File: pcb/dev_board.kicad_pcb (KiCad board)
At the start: 6 copper layers, 45.1 x 41.2 mm, 38 parts, among them J1 Conn_02x13_Odd_Even, J2 Conn_02x13_Odd_Even, J4 Conn_01x05, SW1 SW_DIP_x03, SW2 ARM, U1 LPC, U2 MCP3202, U3 TLV75530PDBV, U6 TLV74311

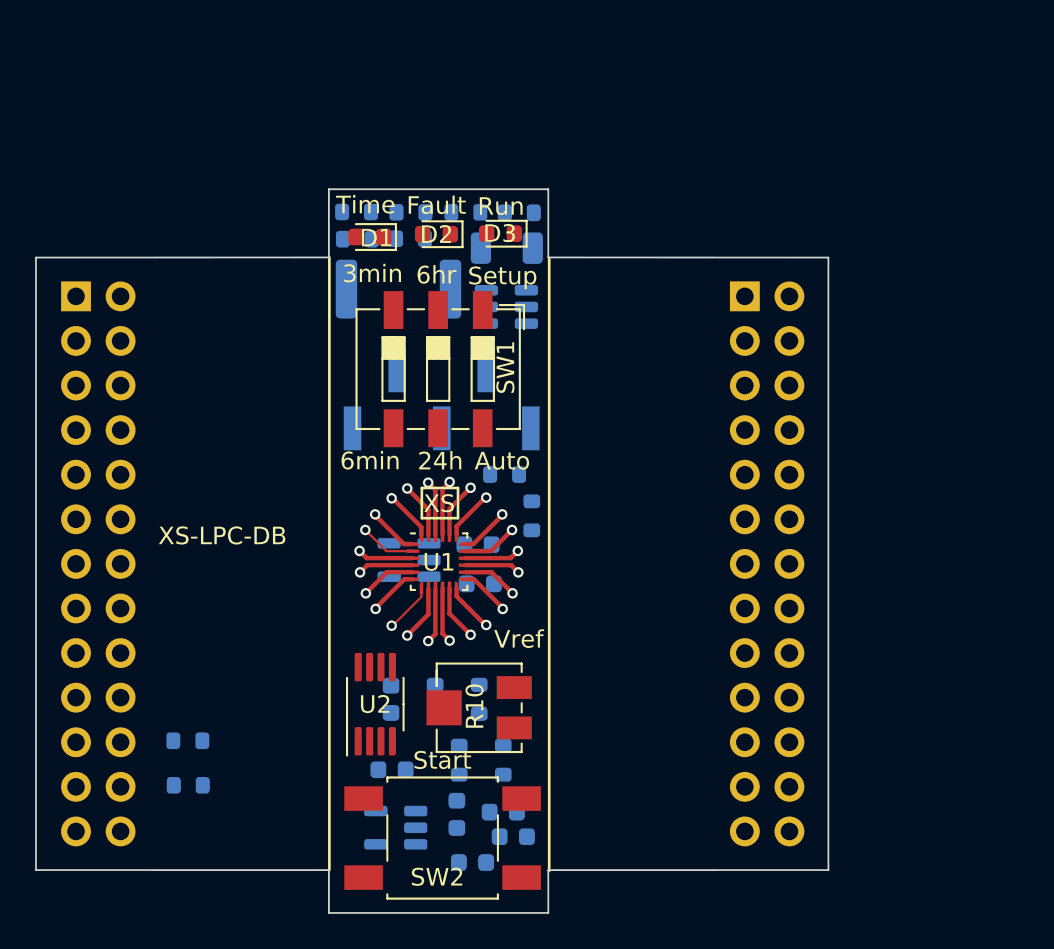
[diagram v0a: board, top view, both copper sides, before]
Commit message: V0.2 schem, bom, pcb. Ready to route
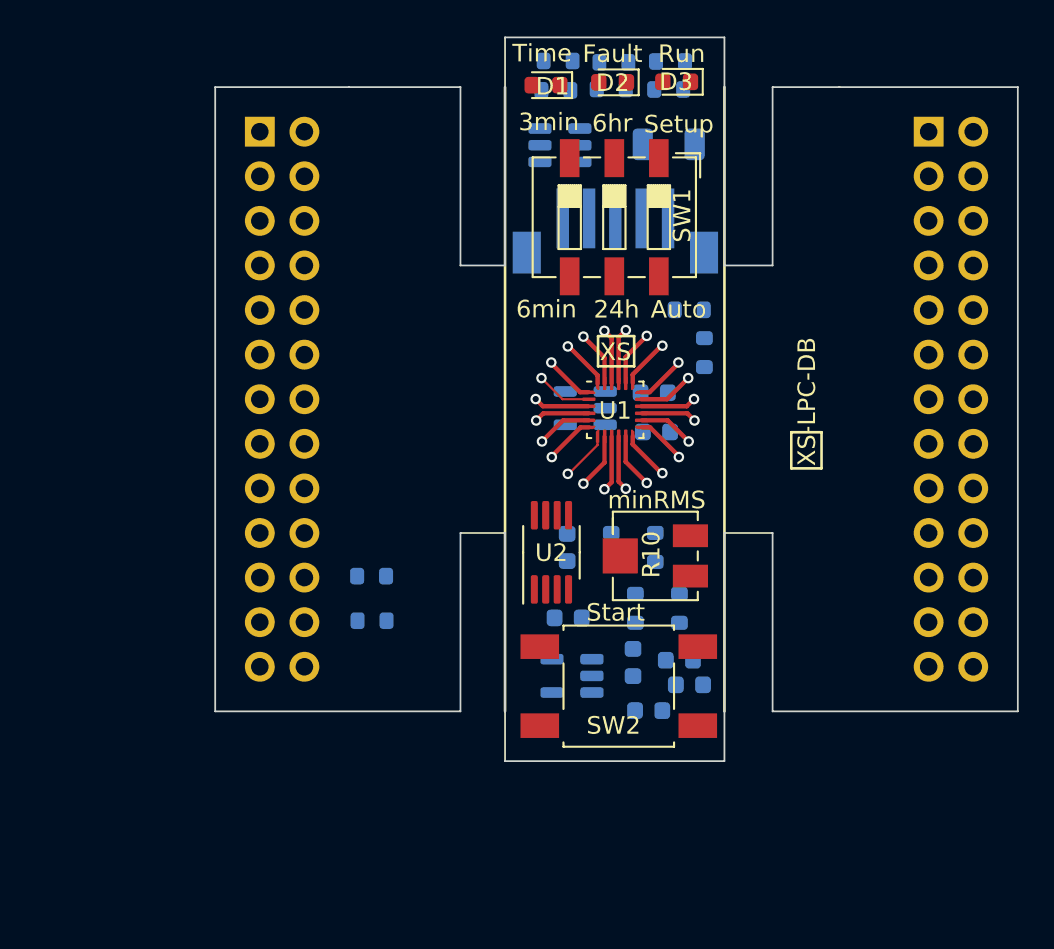
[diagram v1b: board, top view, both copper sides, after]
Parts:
- removed R15: 1R 3W 0.1%, Resistor_SMD:R_2512_6332Metric
- J4: footprint Connector_PinHeader_2.54mm:PinHeader_1x05_P2.54mm_Vertical_SMD_Pin1Left -> Connector_JST:CONN_B5B-ZR-SM4-TF_JST
- R10, R7: value 1K5 -> 1K
- R8: value 18R6 -> 47
- SW2: value ARM -> Start
- U1: value LPC -> XS-LPC-01
- U3: value TLV75530PDBV -> NCP114ASN280T1G
- moved R16 17.0 mm to (173.2, 86.5)
- moved R13 16.8 mm to (169.9, 86.5)
- moved R6 14.1 mm to (174.3, 99.0), turned to 0 degrees
- moved J2 14.1 mm to (149.9, 88.9)
- moved R5 14.1 mm to (156.2, 114.2)
- moved J1 14.1 mm to (188.0, 88.9)
- moved R1 14.1 mm to (156.3, 116.8)
- moved R9 13.5 mm to (175.2, 101.5)
- moved J4 13.5 mm to (170.1, 94.9), turned to 0 degrees
- moved R14 13.3 mm to (166.7, 86.5)
- moved C3 13.2 mm to (173.8, 119.0)
- moved C4 13.2 mm to (172.0, 121.9)
- moved D3 13.2 mm to (173.6, 86.1)
- moved R10 13.2 mm to (172.4, 113.1)
- moved R12 13.2 mm to (173.8, 116.0)
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- renumbered J2 to J1, J1 to J2
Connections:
- J1 pad 10: GND -> /spi_si
- J1 pad 11: /timeout -> GND
- J1 pad 12: GND -> /spi_ss
- J1 pad 13: /time_led -> GND
- J1 pad 14: GND -> /spi_ck
- J1 pad 15: Net-(J2-Pin_15) -> GND
- J1 pad 16: GND -> /osc
- J1 pad 17: Net-(J2-Pin_17) -> GND
- J1 pad 18: GND -> /pump
- J1 pad 19: /adc_clk -> GND
- J1 pad 20: GND -> /start
- J1 pad 21: /adc_miso -> GND
- J1 pad 23: /adc_mosi -> GND
- J1 pad 24: GND -> Net-(J1-Pin_24)
- J1 pad 25: /adc_ncs -> GND
- J1 pad 26: GND -> /sleep_n
- J1 pad 3: unconnected-(J2-Pin_3-Pad3) -> GND
- J1 pad 4: GND -> +3.3V
- J1 pad 5: /setup -> GND
- J1 pad 6: GND -> /run_led
- J1 pad 7: /fault_led -> GND
- J1 pad 8: GND -> /spi_so
- J1 pad 9: /period -> GND
- J2 pad 10: /spi_si -> GND
- J2 pad 11: GND -> /timeout
- J2 pad 12: /spi_ss -> GND
- J2 pad 13: GND -> /time_led
- J2 pad 14: /spi_ck -> GND
- J2 pad 15: GND -> Net-(J2-Pin_15)
- J2 pad 16: /osc -> GND
- J2 pad 17: GND -> Net-(J2-Pin_17)
- J2 pad 18: /pump -> GND
- J2 pad 19: GND -> /adc_clk
- J2 pad 20: /start -> GND
- J2 pad 21: GND -> /adc_miso
- J2 pad 23: GND -> /adc_mosi
- J2 pad 24: Net-(J1-Pin_24) -> GND
- J2 pad 25: GND -> /adc_ncs
- J2 pad 26: /sleep_n -> GND
- J2 pad 3: GND -> unconnected-(J2-Pin_3-Pad3)
- J2 pad 4: +3.3V -> GND
- J2 pad 5: GND -> /setup
- J2 pad 6: /run_led -> GND
- J2 pad 7: GND -> /fault_led
- J2 pad 8: /spi_so -> GND
- J2 pad 9: GND -> /period
- R8 pad 1: /CT1 -> /CT2
- R8 pad 2: /CT2 -> /CT1
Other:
- board size 45.1 x 41.2 mm -> 45.7 x 41.2 mm
- board text added: "minRMS"
- board text removed: "Vref"
